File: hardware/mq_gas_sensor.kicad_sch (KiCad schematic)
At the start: 2 parts, among them U4 MQ-x

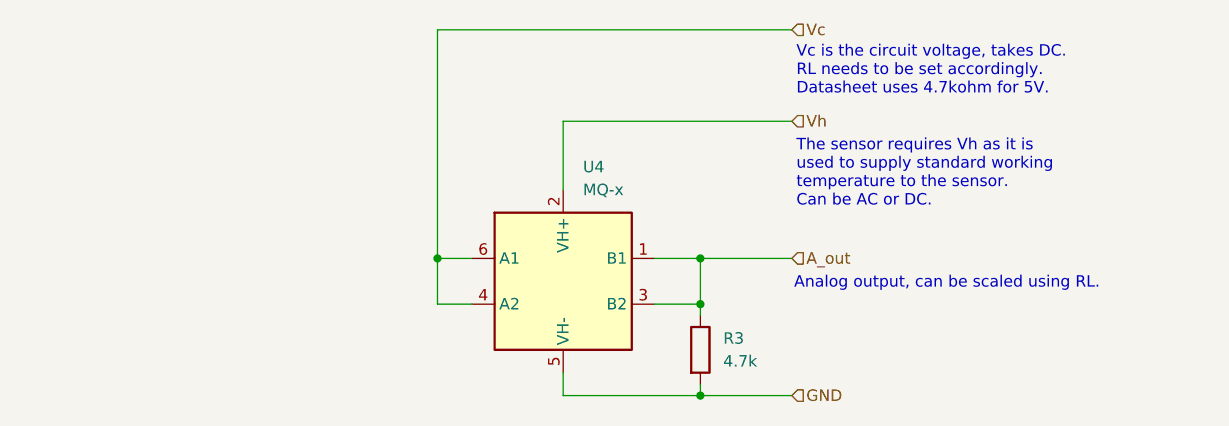
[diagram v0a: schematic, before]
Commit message: completed schematic
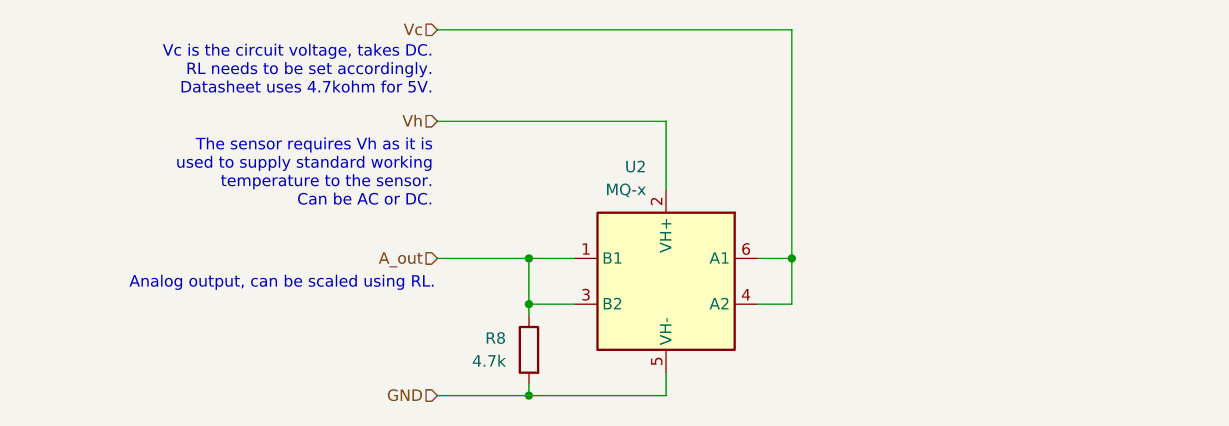
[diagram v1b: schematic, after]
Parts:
- renumbered R3 to R8, U4 to U2
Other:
- moved on the sheet: R8, U2
